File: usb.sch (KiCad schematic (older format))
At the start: 92 parts, among them J201 USB_B, J202 CONN_ICSP, J203 CONN_MRESET, J204 CONN_LED, SW201 SW_RESET, U201 ATmega32U4-AU, U202 MAX7221, Y201 16M, Y202 16M

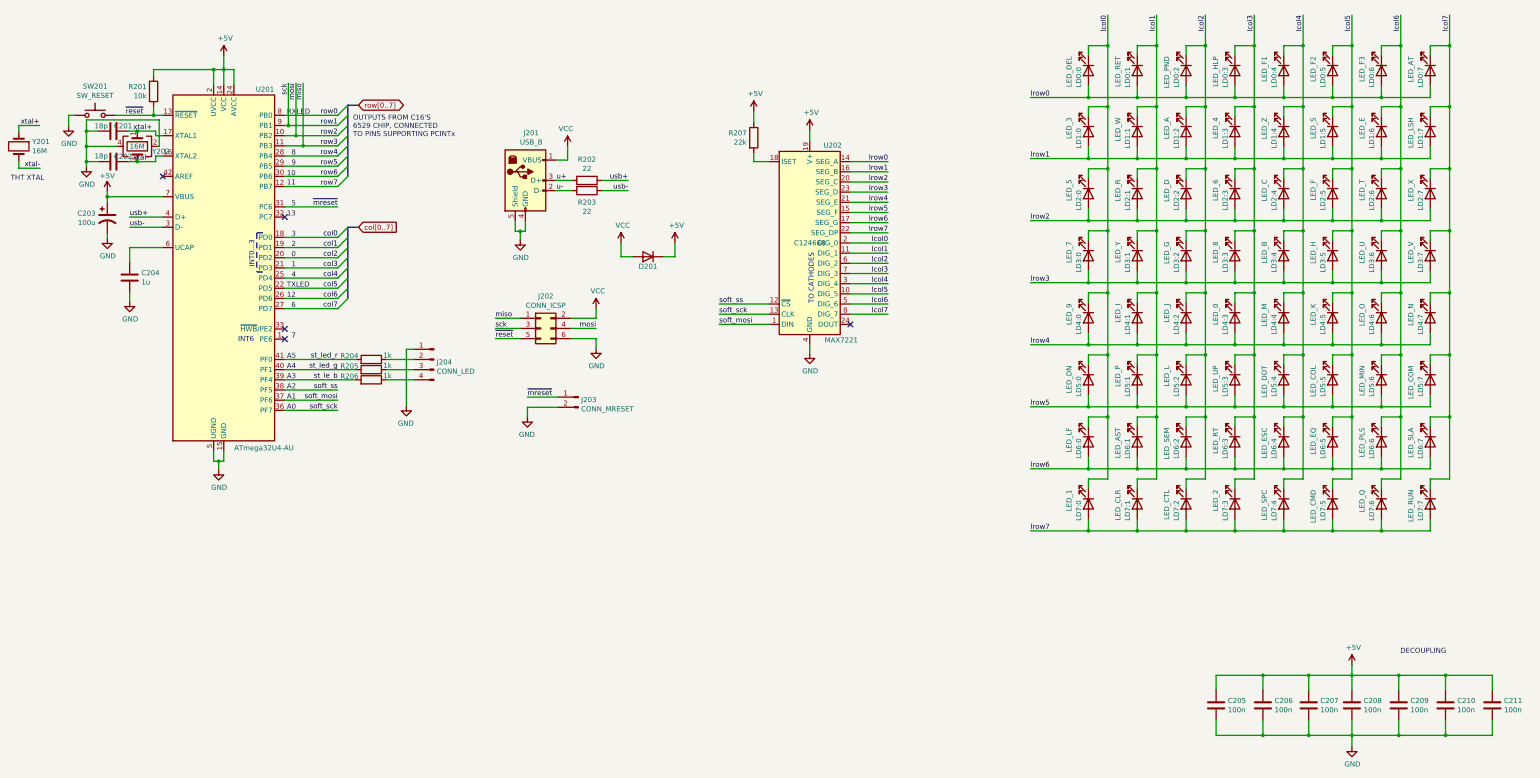
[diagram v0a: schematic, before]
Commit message: Happy?
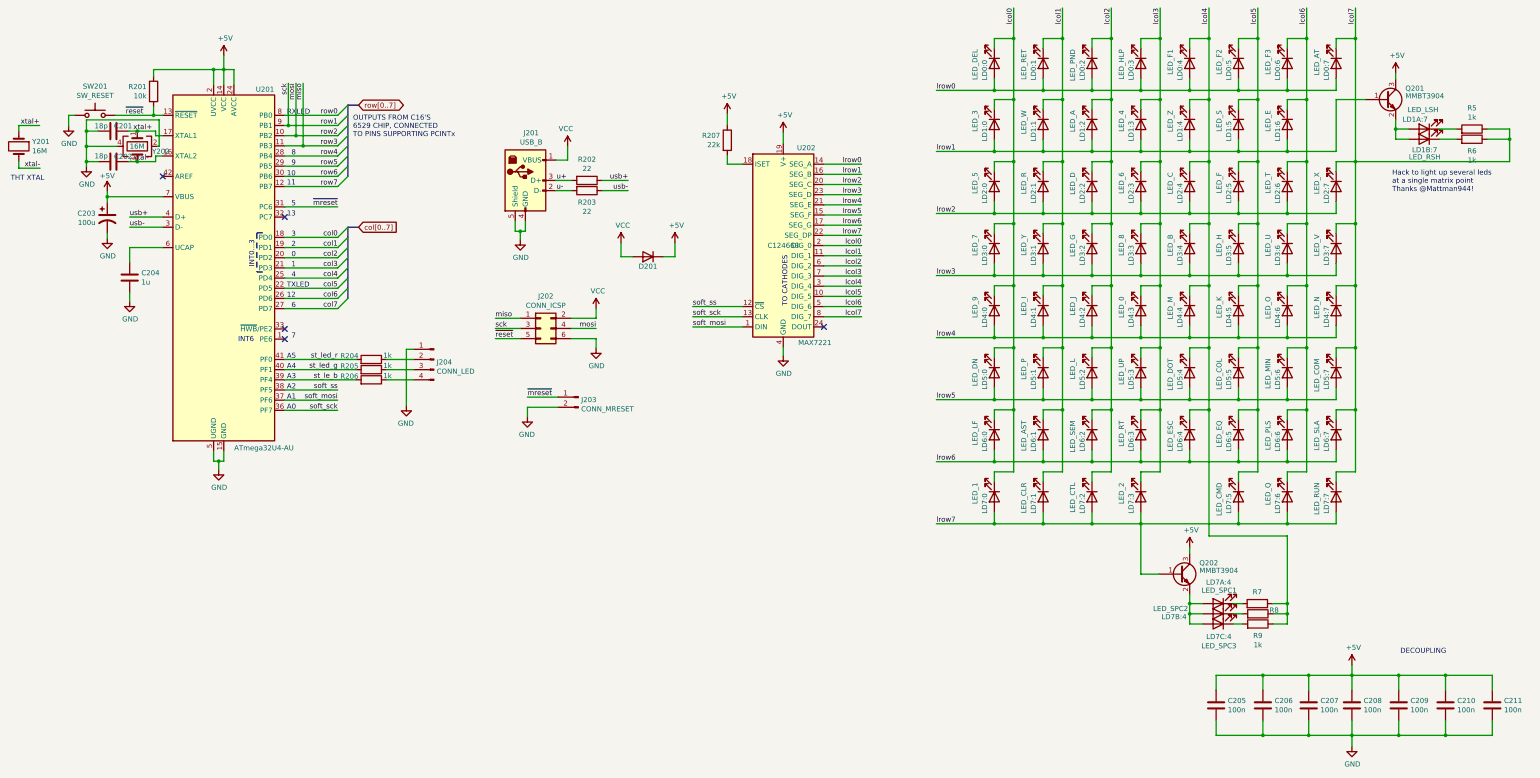
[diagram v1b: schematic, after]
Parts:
- removed LD7:4: LED_SPC, LED_THT:LED_D3.0mm, symbol Device:LED
- added LD1B:7: LED_RSH, LED_THT:LED_D3.0mm, symbol Device:LED
- added LD7A:4: LED_SPC1, LED_THT:LED_D3.0mm, symbol Device:LED
- added LD7B:4: LED_SPC2, LED_THT:LED_D3.0mm, symbol Device:LED
- added LD7C:4: LED_SPC3, LED_THT:LED_D3.0mm, symbol Device:LED
- added Q201, Q202: MMBT3904, Package_TO_SOT_SMD:SOT-23, symbol Device:Q_NPN_BEC
- added R5, R6, R7, R8, R9: 1k, Resistor_SMD:R_0805_2012Metric_Pad1.20x1.40mm_HandSolder, symbol Device:R
- renumbered LD1:7 to LD1A:7
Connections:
- net +5V: now also Q201.3 (C), Q202.3 (C)
- net lcol4: now also R7.1, R8.1, R9.1
- net lcol7: now also R5.1, R6.1; no longer LD1A:7.1 (K)
- net lrow1: now also Q201.1 (B); no longer LD1A:7.2 (A)
- net lrow7: now also Q202.1 (B)
- new net: LD1B:7.1 (K), R6.2
- new net: LD1A:7.2 (A), LD1B:7.2 (A), Q201.2 (E)
- new net: LD1A:7.1 (K), R5.2
- new net: LD7A:4.1 (K), R7.2
- new net: LD7A:4.2 (A), LD7B:4.2 (A), LD7C:4.2 (A), Q202.2 (E)
- new net: LD7B:4.1 (K), R8.2
- new net: LD7C:4.1 (K), R9.2
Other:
- note added: "Hack to light up several leds\nat a single matrix point\nThanks @Mattman944!"
- moved on the sheet: LD0:0, LD0:1, LD0:2, LD0:3, LD0:4, LD0:5, LD0:6, LD0:7, LD1:0, LD1:1, LD1:2, LD1:3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
